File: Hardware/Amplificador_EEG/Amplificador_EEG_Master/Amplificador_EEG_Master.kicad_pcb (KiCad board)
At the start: 2 copper layers, 41 x 49.2 mm, 21 parts, among them J1 VIN, J2 LM385, J3 Coupling_VIN, J4 IN+, J5 IN-, J6 REF, J7 OUTPUT, J8 Mounting_Hole, U1 AD620

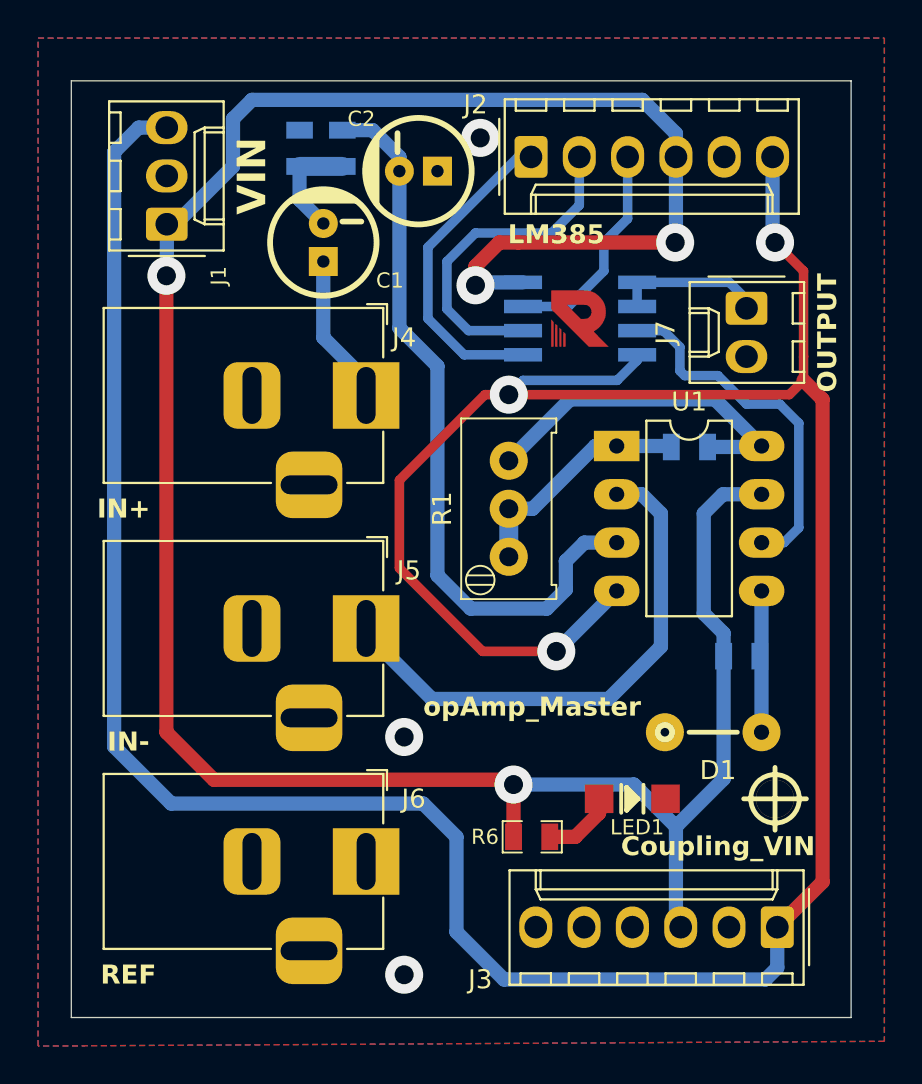
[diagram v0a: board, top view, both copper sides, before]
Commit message: Add files via upload
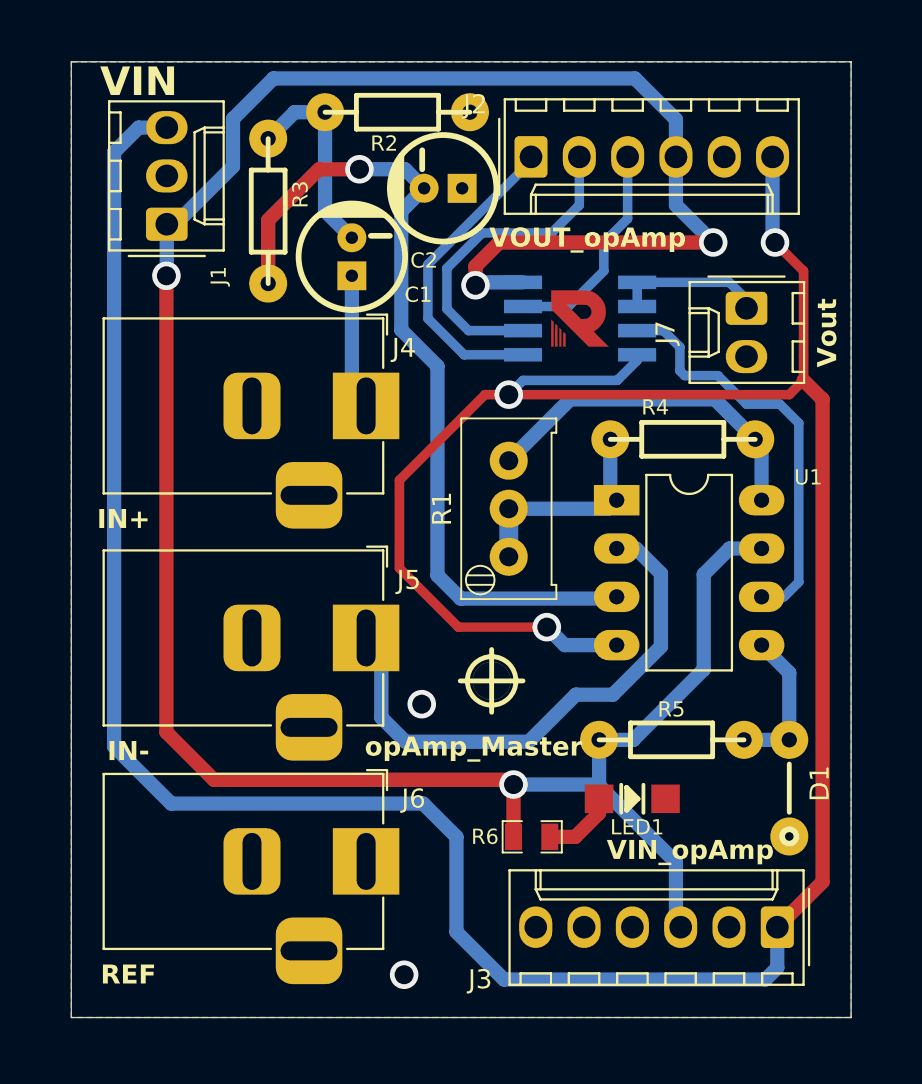
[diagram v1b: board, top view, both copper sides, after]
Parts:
- J2: value LM385 -> VOUT_opAmp
- J3: value Coupling_VIN -> VIN_opAmp
- J7: value OUTPUT -> Vout
- R2, R3, R4, R5: footprint EESTN5:R_0805 -> EESTN5:RES0.3; moved to F.Cu
- moved J8 16.1 mm to (152.3, 110.3)
- moved R5 5.74 mm to (161.8, 113.4)
- moved R2 5.49 mm to (147.4, 80.4), turned to 0 degrees
- moved R3 5.11 mm to (140.6, 85.6), turned to -90 degrees
- moved D1 4.96 mm to (168.0, 115.9), turned to 90 degrees
- moved U1 2.85 mm to (158.9, 100.8)
- moved C1 1.68 mm to (145.0, 88.0)
- moved C2 1.58 mm to (149.8, 84.4)
- moved J4 0.55 mm to (145.8, 95.8)
- moved R4 0.53 mm to (162.4, 97.6)
- moved J5 0.50 mm to (145.8, 108.0)
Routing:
- net /+IN_Clean: track 38.9 -> 45.1 mm, vias 0 -> 1
- net Net-(C1-Pad2): track 5.77 -> 10.7 mm
- net /Vout_AD620: track 19.0 -> 21.9 mm
- net -5V: track 172.8 -> 171.3 mm
- net /Vref: track 7.43 -> 8.65 mm
- net /IN-: track 27.8 -> 28.8 mm
- net Net-(R1-Pad1): track 12.9 -> 12.1 mm
- net GND: vias 3 -> 2
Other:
- board size 41 x 49.2 mm -> 41 x 50.2 mm

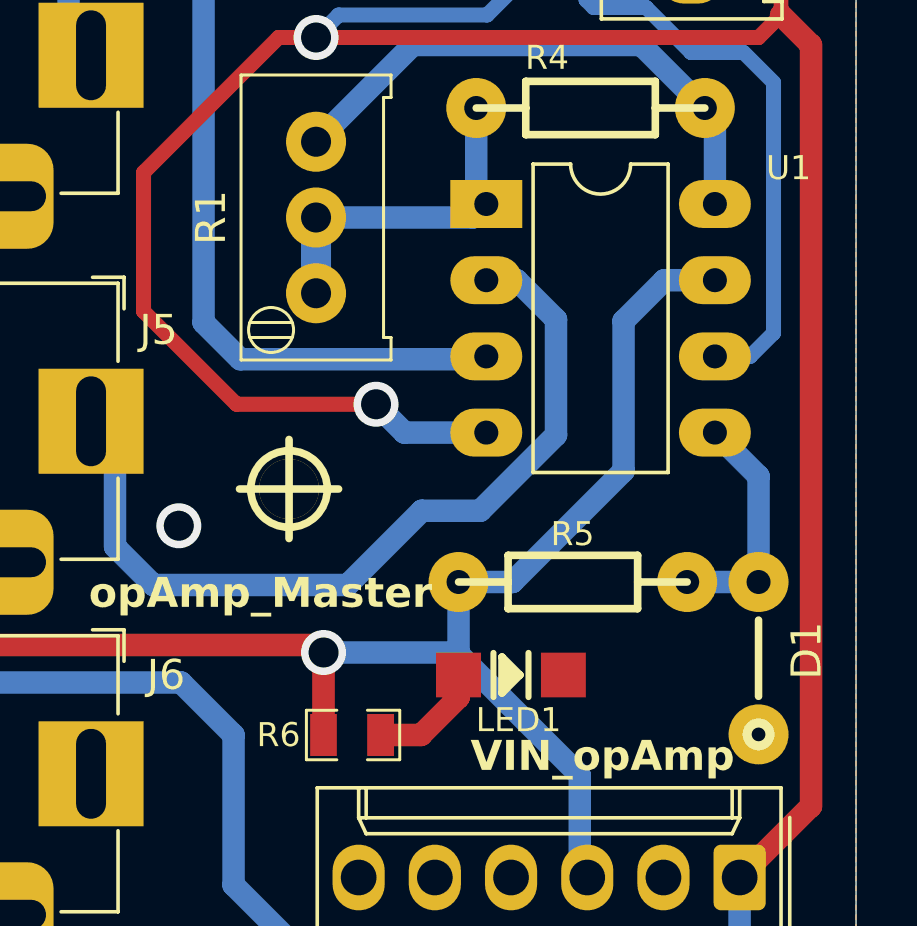
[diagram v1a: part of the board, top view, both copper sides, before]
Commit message: Add files via upload
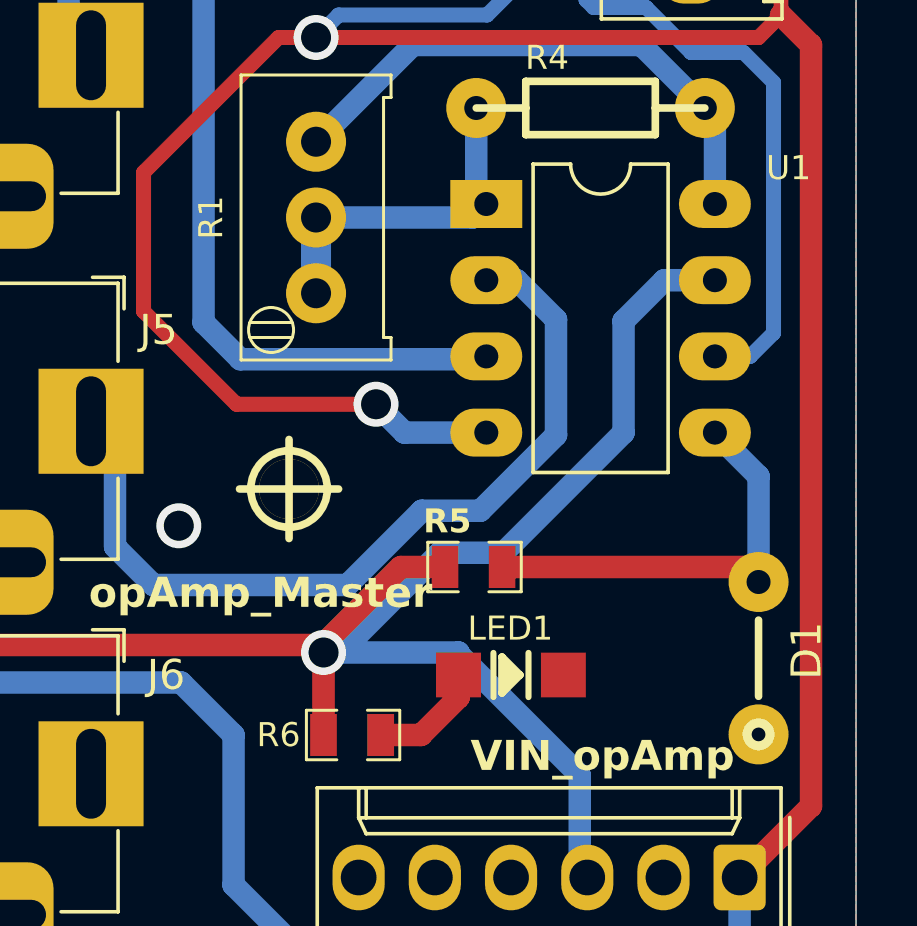
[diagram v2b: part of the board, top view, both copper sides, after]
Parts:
- R5: footprint EESTN5:RES0.3 -> EESTN5:R_0805
- moved R5 3.35 mm to (158.5, 112.9)
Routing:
- net +5V: track 136.8 -> 144.6 mm
- net /Vref: track 8.65 -> 15.0 mm
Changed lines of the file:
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@@
 		)
 		(property "Value" "2,2k"
-			(at 0 2.032 360)
+			(at 0 2.032 0)
 			(layer "F.SilkS")
 			(hide yes)
@@
 		)
 		(property "Footprint" "EESTN5:RES0.3"
-			(at 0 0 360)
+			(at 0 0 0)
 			(layer "F.Fab")
 			(hide yes)
@@
 		)
 		(property "Datasheet" ""
-			(at 0 0 360)
+			(at 0 0 0)
 			(layer "F.Fab")
 			(hide yes)
@@
 		)
 		(property "Description" "Resistor"
-			(at 0 0 360)
+			(at 0 0 0)
 			(layer "F.Fab")
 			(hide yes)
@@
 		(descr "SMD LED_ 1206")
 		(property "Reference" "LED1"
-			(at 0.25248 1.5 0)
+			(at -0.02252 -1.55 0)
 			(layer "F.SilkS")
 			(effects
@@
 		)
 		(property "Value" "2,7k"
-			(at 0 2.032 360)
+			(at 0 2.032 0)
 			(layer "F.SilkS")
 			(hide yes)
@@
 		)
 		(property "Footprint" "EESTN5:RES0.3"
-			(at 0 0 360)
+			(at 0 0 0)
 			(layer "F.Fab")
 			(hide yes)
@@
 		)
 		(property "Datasheet" ""
-			(at 0 0 360)
+			(at 0 0 0)
 			(layer "F.Fab")
 			(hide yes)
@@
 		)
 		(property "Description" "Resistor"
-			(at 0 0 360)
+			(at 0 0 0)
 			(layer "F.Fab")
 			(hide yes)
@@
 			(effects
 				(font
-					(size 1 1)
-					(thickness 0.1)
+					(size 0.8 0.8)
+					(thickness 0.15)
 				)
 			)
@@
 		)
 	)
-	(footprint "EESTN5:RES0.3"
+	(footprint "EESTN5:R_0805"
 		(layer "F.Cu")
-		(at 161.81 113.4)
-		(descr "Resistor, RC03")
-		(tags "R")
+		(at 158.5 112.9)
 		(property "Reference" "R5"
-			(at -0.01 -1.6 0)
+			(at -0.875 -1.525 0)
 			(layer "F.SilkS")
 			(effects
 				(font
 					(size 0.8 0.8)
-					(thickness 0.2)
+					(thickness 0.15)
+					(bold yes)
 				)
 			)
 		)
 		(property "Value" "330"
-			(at 0 2.032 360)
+			(at 0 2.1 0)
 			(layer "F.SilkS")
 			(hide yes)
@@
 			)
 		)
-		(property "Footprint" "EESTN5:RES0.3"
-			(at 0 0 360)
+		(property "Footprint" "EESTN5:R_0805"
+			(at 0 0 0)
 			(layer "F.Fab")
 			(hide yes)
@@
 		)
 		(property "Datasheet" ""
-			(at 0 0 360)
+			(at 0 0 0)
 			(layer "F.Fab")
 			(hide yes)
@@
 		)
 		(property "Description" "Resistor"
-			(at 0 0 360)
+			(at 0 0 0)
 			(layer "F.Fab")
 			(hide yes)
@@
 		(sheetname "Raíz")
 		(sheetfile "Amplificador_EEG_Master.kicad_sch")
-		(attr through_hole)
+		(attr smd)
 		(fp_line
-			(start -2.159 -0.889)
-			(end -2.159 0.889)
+			(start -1.524 -0.8255)
+			(end -0.508 -0.8255)
 			(stroke
-				(width 0.254)
+				(width 0.09906)
 				(type solid)
 			)
@@
 		)
 		(fp_line
-			(start -2.159 0)
-			(end -3.81 0)
+			(start -1.524 0.8255)
+			(end -1.524 -0.8255)
 			(stroke
-				(width 0.254)
+				(width 0.09906)
 				(type solid)
 			)
@@
 		)
 		(fp_line
-			(start -2.159 0.889)
-			(end 2.159 0.889)
+			(start -0.508 0.8255)
+			(end -1.524 0.8255)
 			(stroke
-				(width 0.254)
+				(width 0.09906)
 				(type solid)
 			)
@@
 		)
 		(fp_line
-			(start 2.159 -0.889)
-			(end -2.159 -0.889)
+			(start 0.508 -0.8255)
+			(end 1.5875 -0.8255)
 			(stroke
-				(width 0.254)
+				(width 0.09906)
 				(type solid)
 			)
@@
 		)
 		(fp_line
-			(start 2.159 0)
-			(end 3.81 0)
+			(start 1.5875 -0.8255)
+			(end 1.5875 0.8255)
 			(stroke
-				(width 0.254)
+				(width 0.09906)
 				(type solid)
 			)
@@
 		)
 		(fp_line
-			(start 2.159 0.889)
-			(end 2.159 -0.889)
+			(start 1.5875 0.8255)
+			(end 0.508 0.8255)
 			(stroke
-				(width 0.254)
+				(width 0.09906)
 				(type solid)
 			)
 			(layer "F.SilkS")
 		)
-		(pad "1" thru_hole circle
-			(at -3.81 0)
-			(size 1.99898 1.99898)
-			(drill 0.8001)
-			(layers "*.Cu" "*.Mask" "F.SilkS")
-			(remove_unused_layers no)
+		(pad "1" smd rect
+			(at -0.9525 0)
+			(size 0.889 1.397)
+			(layers "F.Cu" "F.Paste" "F.Mask")
 			(net 5 "+5V")
 			(pintype "passive")
 		)
-		(pad "2" thru_hole circle
-			(at 3.81 0)
-			(size 1.99898 1.99898)
-			(drill 0.8001)
-			(layers "*.Cu" "*.Mask" "F.SilkS")
-			(remove_unused_layers no)
+		(pad "2" smd rect
+			(at 0.9525 0)
+			(size 0.889 1.397)
+			(layers "F.Cu" "F.Paste" "F.Mask")
 			(net 17 "/Vref")
 			(pintype "passive")
 		)
-		(model "res0.3.wrl"
+		(model "${KISYS3DMOD}/R_0805.wrl"
 			(offset
-				(xyz 1.523999977 0 1.015999985)
+				(xyz 0 0 0)
 			)
 			(scale
-				(xyz 0.393701 0.393701 0.393701)
+				(xyz 1 1 1)
 			)
 			(rotate
-				(xyz -90 0 90)
+				(xyz 0 0 0)
 			)
 		)
@@
 	)
 	(segment
+		(start 156.075 112.9)
+		(end 157.5475 112.9)
+		(width 0.75)
+		(layer "F.Cu")
+		(net 5)
+	)
+	(segment
 		(start 151.5 88.5)
 		(end 151.5 89.5)
@@
 	)
 	(segment
+		(start 153.5 115.75)
+		(end 153.5 115.475)
+		(width 0.75)
+		(layer "F.Cu")
+		(net 5)
+	)
+	(segment
 		(start 137.75 115.5)
 		(end 153.25 115.5)
@@
 	)
 	(segment
+		(start 153.5 115.475)
+		(end 156.075 112.9)
+		(width 0.75)
+		(layer "F.Cu")
+		(net 5)
+	)
+	(segment
 		(start 153.25 115.5)
 		(end 153.5 115.75)
@@
 	)
 	(segment
-		(start 138.75 80.75)
-		(end 140.875 78.625)
+		(start 157.375 112.425)
+		(end 154.05 115.75)
 		(width 0.75)
 		(layer "B.Cu")
@@
 	)
 	(segment
-		(start 162.04 80.78)
-		(end 162.04 82.75)
+		(start 138.75 80.75)
+		(end 140.875 78.625)
 		(width 0.75)
 		(layer "B.Cu")
@@
 	)
 	(segment
-		(start 158 113.4)
-		(end 158 115.75)
+		(start 162.04 80.78)
+		(end 162.04 82.75)
 		(width 0.75)
 		(layer "B.Cu")
@@
 	)
 	(segment
-		(start 158 113.4)
-		(end 159.8 113.4)
+		(start 135.27 88.98)
+		(end 135.25 89)
 		(width 0.75)
 		(layer "B.Cu")
@@
 	)
 	(segment
-		(start 135.27 88.98)
-		(end 135.25 89)
+		(start 140.875 78.625)
+		(end 159.885 78.625)
+		(width 0.75)
+		(layer "B.Cu")
+		(net 5)
+	)
+	(segment
+		(start 135.27 86.29)
+		(end 135.71 86.29)
 		(width 0.75)
 		(layer "B.Cu")
@@
 	)
 	(segment
-		(start 159.8 113.4)
-		(end 163.5 109.7)
+		(start 164.86 103.34)
+		(end 163.5 104.7)
 		(width 0.75)
 		(layer "B.Cu")
@@
 	(segment
 		(start 163.5 104.7)
-		(end 164.86 103.34)
+		(end 163.5 108.425)
 		(width 0.75)
 		(layer "B.Cu")
@@
 	)
 	(segment
-		(start 140.875 78.625)
-		(end 159.885 78.625)
+		(start 163.5 108.425)
+		(end 159.5 112.425)
 		(width 0.75)
 		(layer "B.Cu")
@@
 	)
 	(segment
-		(start 135.27 86.29)
-		(end 135.71 86.29)
+		(start 159.5 112.425)
+		(end 157.375 112.425)
+		(width 0.75)
+		(layer "B.Cu")
+		(net 5)
+	)
+	(segment
+		(start 154.05 115.75)
+		(end 153.5 115.75)
 		(width 0.75)
 		(layer "B.Cu")
@@
 	)
 	(segment
-		(start 164.86 103.34)
-		(end 166.545 103.34)
+		(start 166.545 103.34)
+		(end 164.86 103.34)
 		(width 0.75)
 		(layer "B.Cu")
@@
 	)
 	(segment
-		(start 163.5 109.7)
-		(end 163.5 104.7)
-		(width 0.75)
-		(layer "B.Cu")
-		(net 5)
-	)
-	(segment
 		(start 135.27 86.29)
 		(end 135.27 88.98)
@@
 	)
 	(segment
-		(start 168 113)
+		(start 167.5 112.9)
 		(end 168 113.4)
 		(width 0.75)
-		(layer "B.Cu")
+		(layer "F.Cu")
 		(net 17)
 	)
 	(segment
-		(start 168 109.875)
-		(end 166.545 108.42)
+		(start 159.4525 112.9)
+		(end 167.5 112.9)
+		(width 0.75)
+		(layer "F.Cu")
+		(net 17)
+	)
+	(segment
+		(start 168 113)
+		(end 168 113.4)
 		(width 0.75)
 		(layer "B.Cu")
@@
 	)
 	(segment
-		(start 168 113.4)
-		(end 165.62 113.4)
+		(start 168 109.875)
+		(end 166.545 108.42)
 		(width 0.75)
 		(layer "B.Cu")
